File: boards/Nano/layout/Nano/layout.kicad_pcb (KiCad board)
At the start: 4 copper layers, 19 x 44 mm, 35 parts, among them IC1 ATMEGA328PMAU, IC2 AMS1117M5_0, IC3 FT231XQMR, J1 2.54mm 15x1, J2 2.54mm 15x1, J3 10033526MN3212LF, J4 2.54mm 3x2, Y1 16MHz 18pF

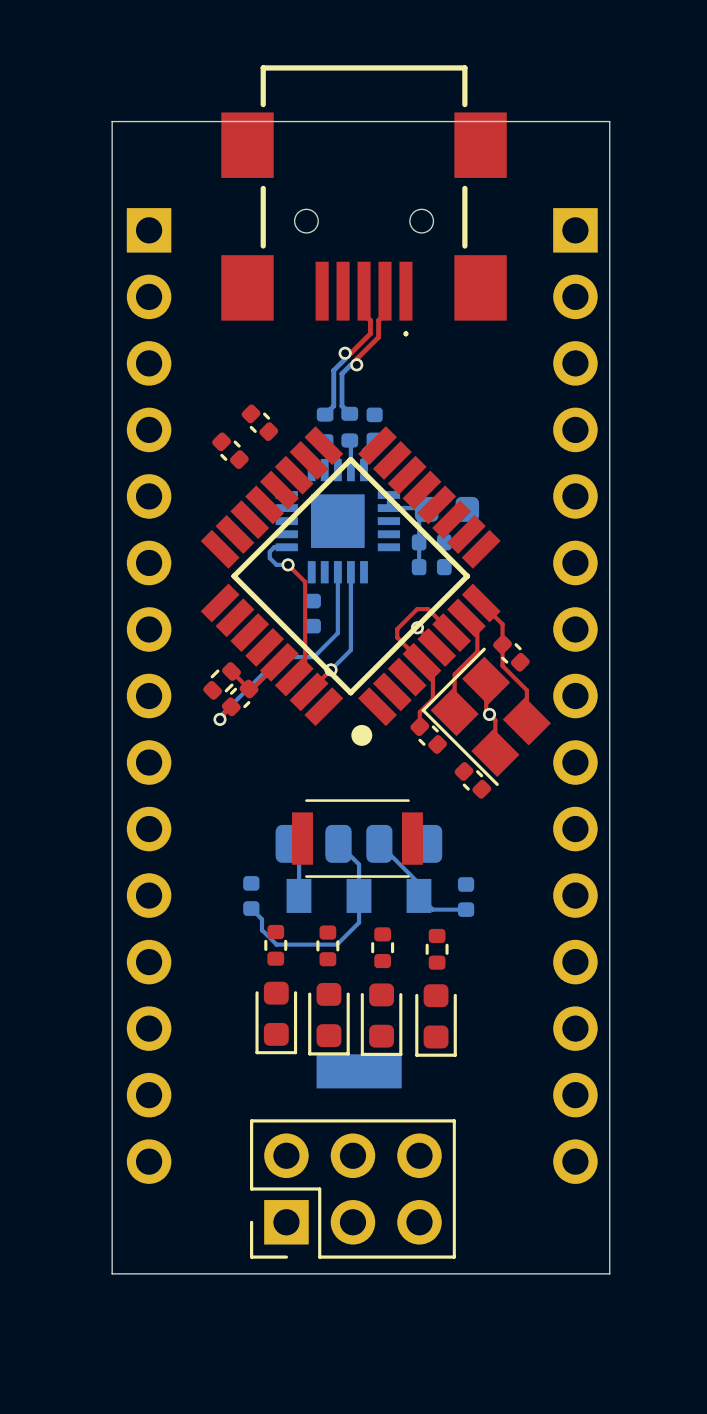
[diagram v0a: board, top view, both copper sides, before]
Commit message: full routing
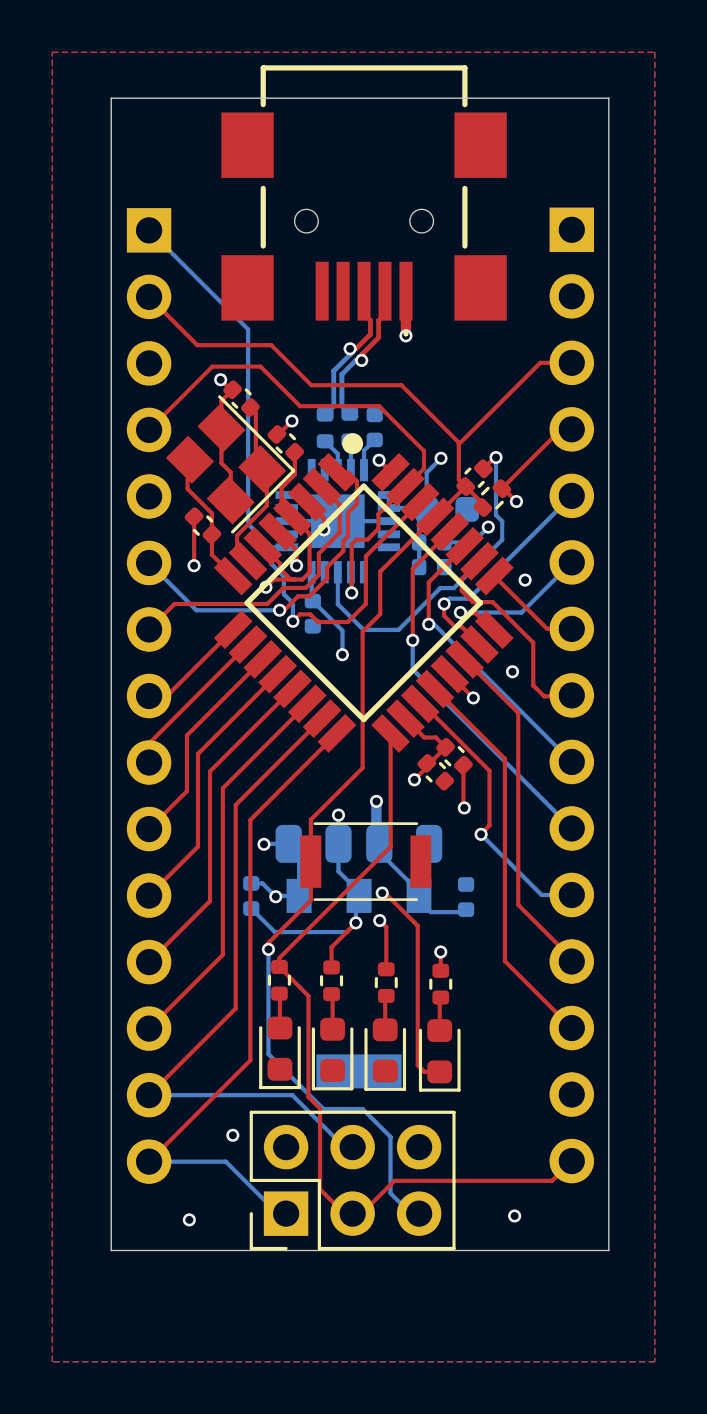
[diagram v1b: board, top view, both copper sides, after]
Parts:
- moved C5 17.0 mm to (67.2, 90.7), turned to 135 degrees
- moved C2 14.7 mm to (75.4, 104.4), turned to -45 degrees
- moved C3 14.6 mm to (74.6, 105.0), turned to -45 degrees
- moved Y1 14.0 mm to (66.6, 93.2), turned to 135 degrees
- moved C6 12.7 mm to (65.8, 95.6), turned to 135 degrees
- moved R1 12.5 mm to (76.8, 94.5), turned to 45 degrees
- moved C4 12.4 mm to (68.9, 92.4), turned to 135 degrees
- moved C1 12.3 mm to (76.1, 93.7), turned to -135 degrees
- moved R2 1.34 mm to (68.7, 112.9)
- moved D1 1.34 mm to (68.7, 115.5)
- moved D2 1.34 mm to (70.7, 115.6)
- moved D3 1.34 mm to (72.7, 115.6)
- moved D4 1.34 mm to (74.8, 115.6)
- moved R3 1.34 mm to (70.7, 113.0)
- moved R4 1.34 mm to (72.8, 113.0)
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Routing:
- net RESET: track 2.53 -> 57.1 mm, vias 0 -> 1
- net UART_TX: track 5.23 -> 42.7 mm, vias 1 -> 2
- net UART_RX: track 6.49 -> 42.0 mm, vias 1 -> 2
- net D13: track 0.00 -> 30.9 mm
- net D11: track 0.00 -> 25.9 mm
- net D12: track 0.00 -> 25.5 mm
- net USB_VBUS: track 4.63 -> 28.0 mm, vias 0 -> 2
- net VCC_5V: track 20.2 -> 39.1 mm, vias 0 -> 8
- net GND: track 6.11 -> 24.3 mm, vias 2 -> 15
- net AREF: track 0.00 -> 15.1 mm
- net D10: track 0.00 -> 14.9 mm
- net A5: track 0.00 -> 14.4 mm, vias 0 -> 1
- net A7: track 0.00 -> 13.3 mm
- net D3: track 0.00 -> 13.1 mm, vias 0 -> 1
- net D9: track 0.00 -> 12.7 mm
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- added copper zone on B.Cu, net GND
- added copper zone on F.Cu, net GND
- added copper zone on In1.Cu, net GND
- added copper zone on In2.Cu, net VCC_5V
